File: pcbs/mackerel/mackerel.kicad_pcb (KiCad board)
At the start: 2 copper layers, 129.5 x 96.8 mm, 60 parts, among them J1 MJ-4PP-9-kbd-corne-light-resc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, SW1 SW_Push, SW10 SW_Push, SW11 SW_Push, SW12 SW_Push, SW13 SW_Push, SW14 SW_Push, SW15 SW_Push, SW16 SW_Push, SW17 SW_Push, SW18 SW_Push, SW19 SW_Push, SW2 SW_Push, SW20 SW_Push, SW21 SW_Push, SW22 SW_Push, SW23 SW_Push, SW24 SW_Push, SW25 SW_Push, SW26 SW_Push, SW27 SW_Push, SW28 SW_Push, SW29 SW_Push, SW3 SW_Push, SW4 SW_Push, SW5 SW_Push, SW6 SW_Push, SW7 SW_Push, SW8 SW_Push, SW9 SW_Push, U1 rp2040-zero

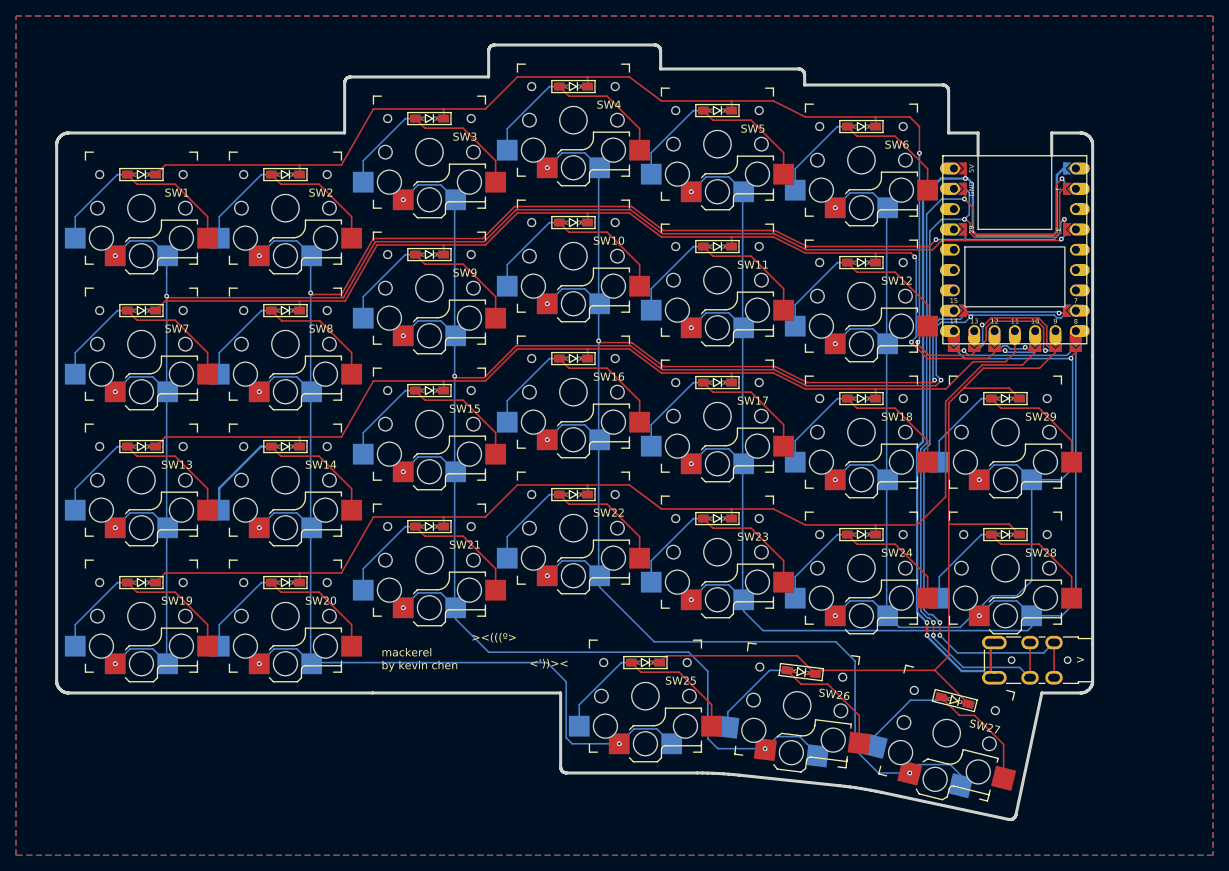
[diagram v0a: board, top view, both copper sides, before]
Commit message: updates
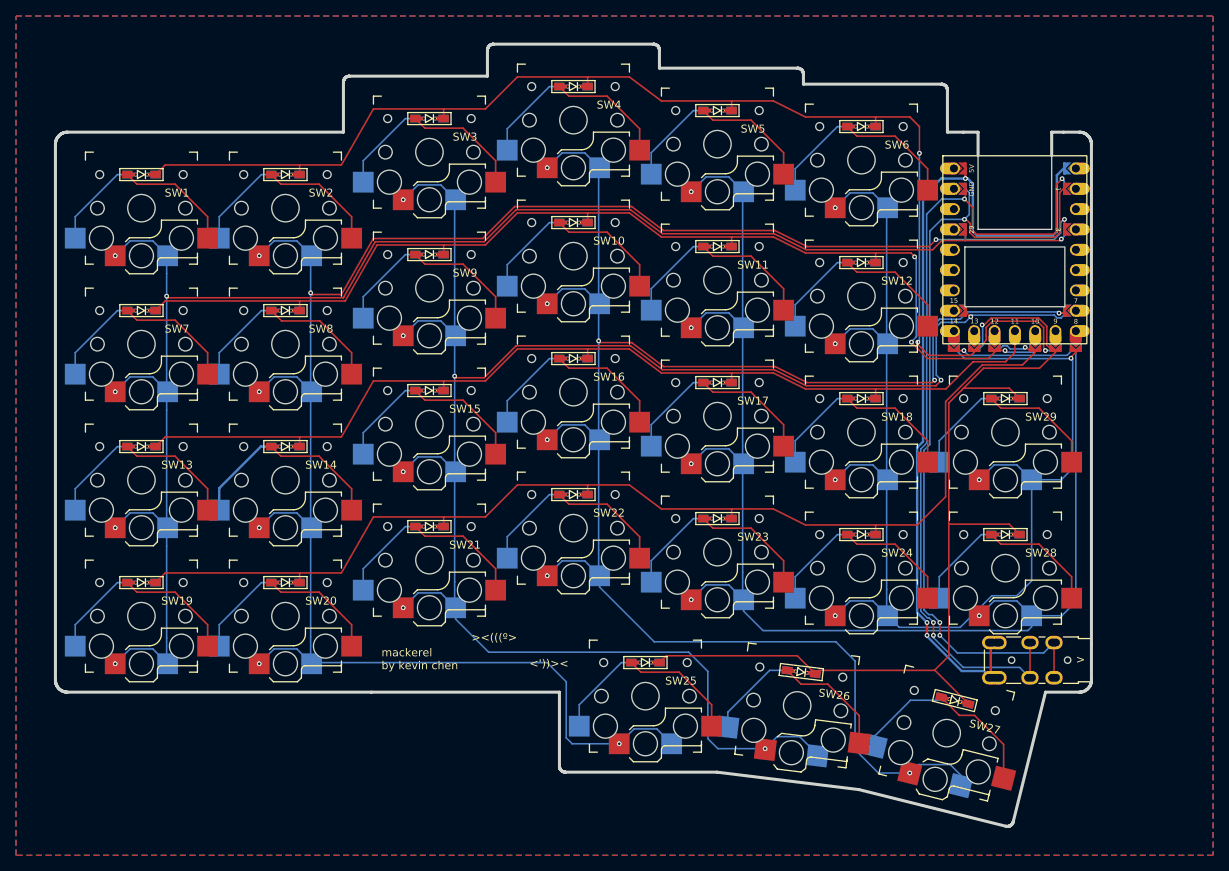
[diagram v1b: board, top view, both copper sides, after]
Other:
- board size 129.5 x 96.8 mm -> 129.5 x 97.8 mm
